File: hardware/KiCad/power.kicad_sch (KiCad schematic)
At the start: 22 parts, among them U4 SCT2A25STER, U5 SY8120B1ABC

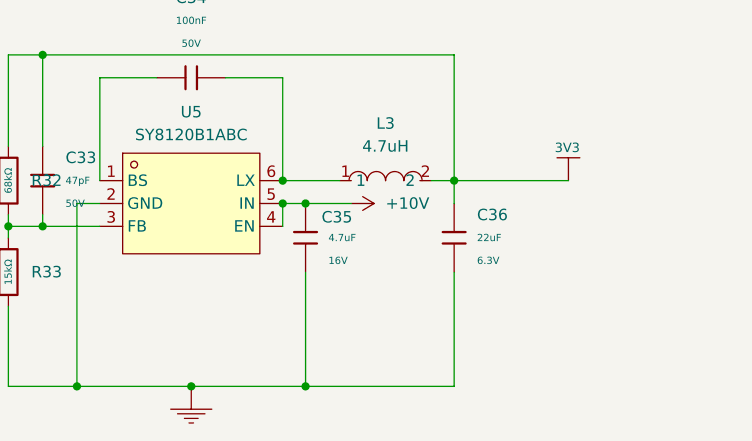
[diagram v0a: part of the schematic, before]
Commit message: changes
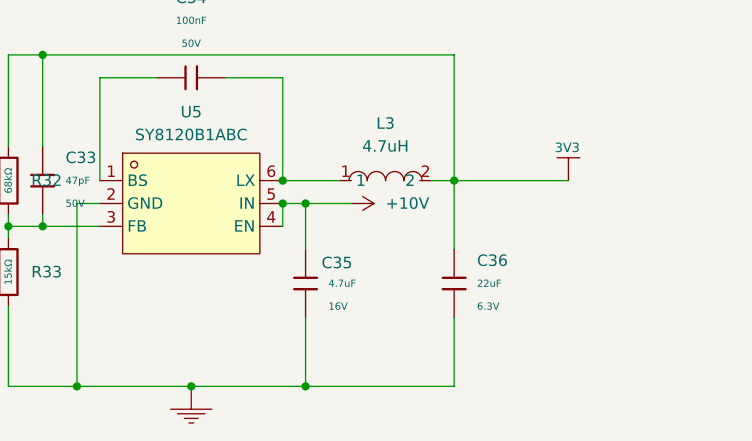
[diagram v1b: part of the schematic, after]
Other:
- moved on the sheet: C35, C36
